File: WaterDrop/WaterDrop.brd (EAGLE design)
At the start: 20 x 35 mm, 12 parts, among them IC1 PIC12F1822

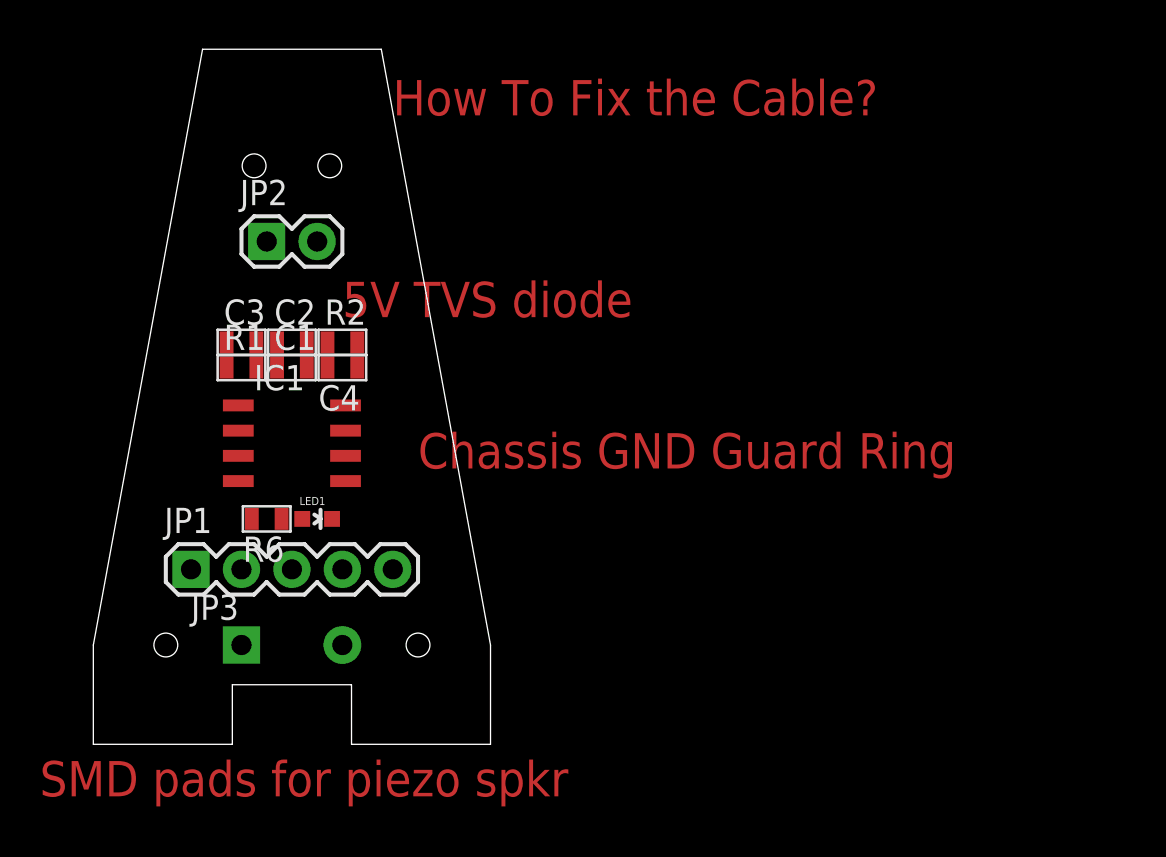
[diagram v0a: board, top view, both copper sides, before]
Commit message: random cotroller added
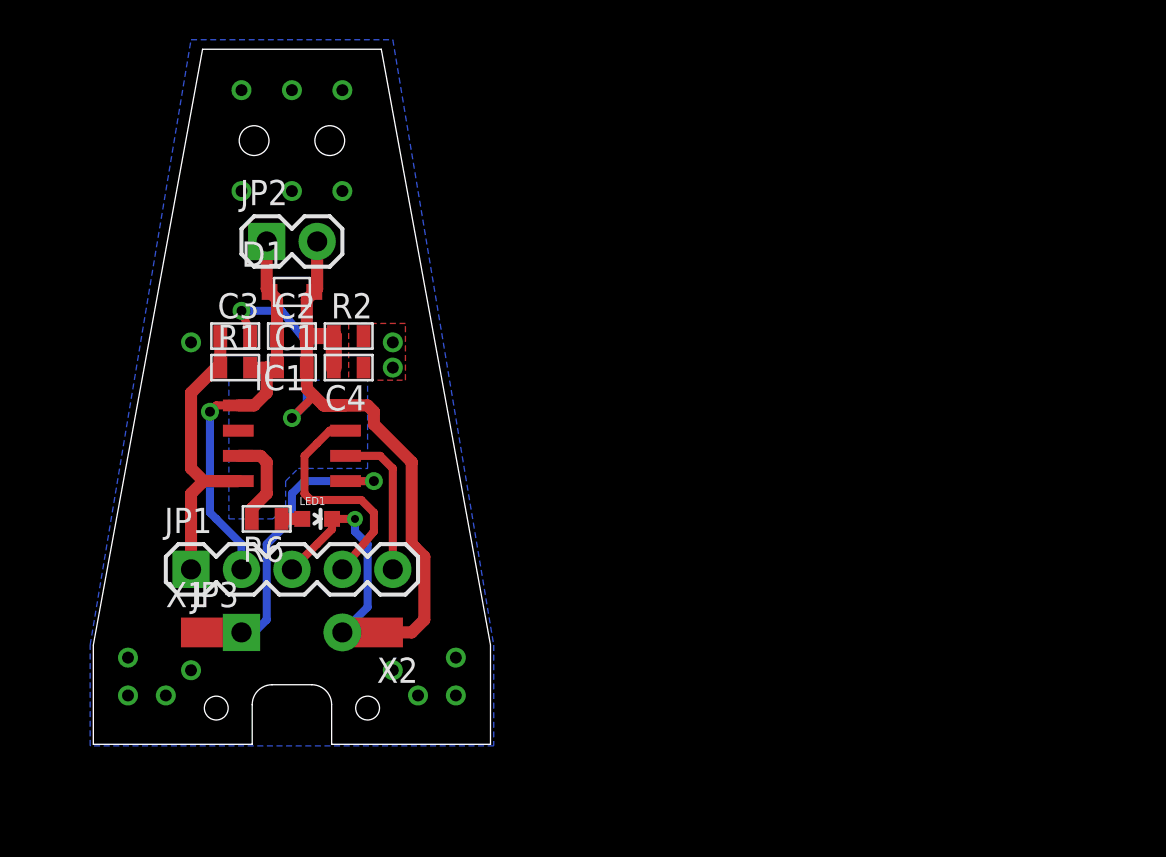
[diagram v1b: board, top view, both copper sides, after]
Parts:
- added D1: SD0, WaterDrop:SOD-323
- added X1, X2: P-PAD-S, OSSI:P-PAD-S
- moved JP3 0.64 mm to (0.00, 0.64)
- moved C3 0.45 mm to (-2.86, 15.6)
- moved R2 0.45 mm to (2.86, 15.6)
- moved C4 0.32 mm to (2.86, 14.0)
- moved R1 0.32 mm to (-2.86, 14.0)
- moved C2 0.32 mm to (0.00, 15.6)
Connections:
- net +5V: now also D1.1
- net GND: now also D1.2, X2.1
- net PIEZO: now also X1.1
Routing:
- net GND: track 0.00 -> 54.9 mm, vias 0 -> 3
- net +5V: track 0.00 -> 21.0 mm, vias 0 -> 1
- net /RST: track 0.00 -> 16.5 mm
- net PIEZO: track 0.00 -> 15.5 mm, vias 0 -> 1
- net ICSPDAT: track 0.00 -> 11.8 mm
- net ICSPCLK: track 0.00 -> 7.72 mm
- net N$3: track 0.00 -> 4.73 mm
- net N$2: track 0.00 -> 1.04 mm
- added copper zone on layer 16, net N$1
- added copper zone on layer 1, net STRUT_GND
- added copper zone on layer 16, net STRUT_GND
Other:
- outline, holes or cut-outs redrawn
- board text removed: "5V TVS diode"
- board text removed: "Chassis GND Guard Ring"
- board text removed: "How To Fix the Cable?"
- board text removed: "SMD pads for piezo spkr"
